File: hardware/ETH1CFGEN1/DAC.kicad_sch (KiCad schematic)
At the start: 42 parts, among them U601 TL072CD, U602 DAC8568IBPW, U603 TL072CD

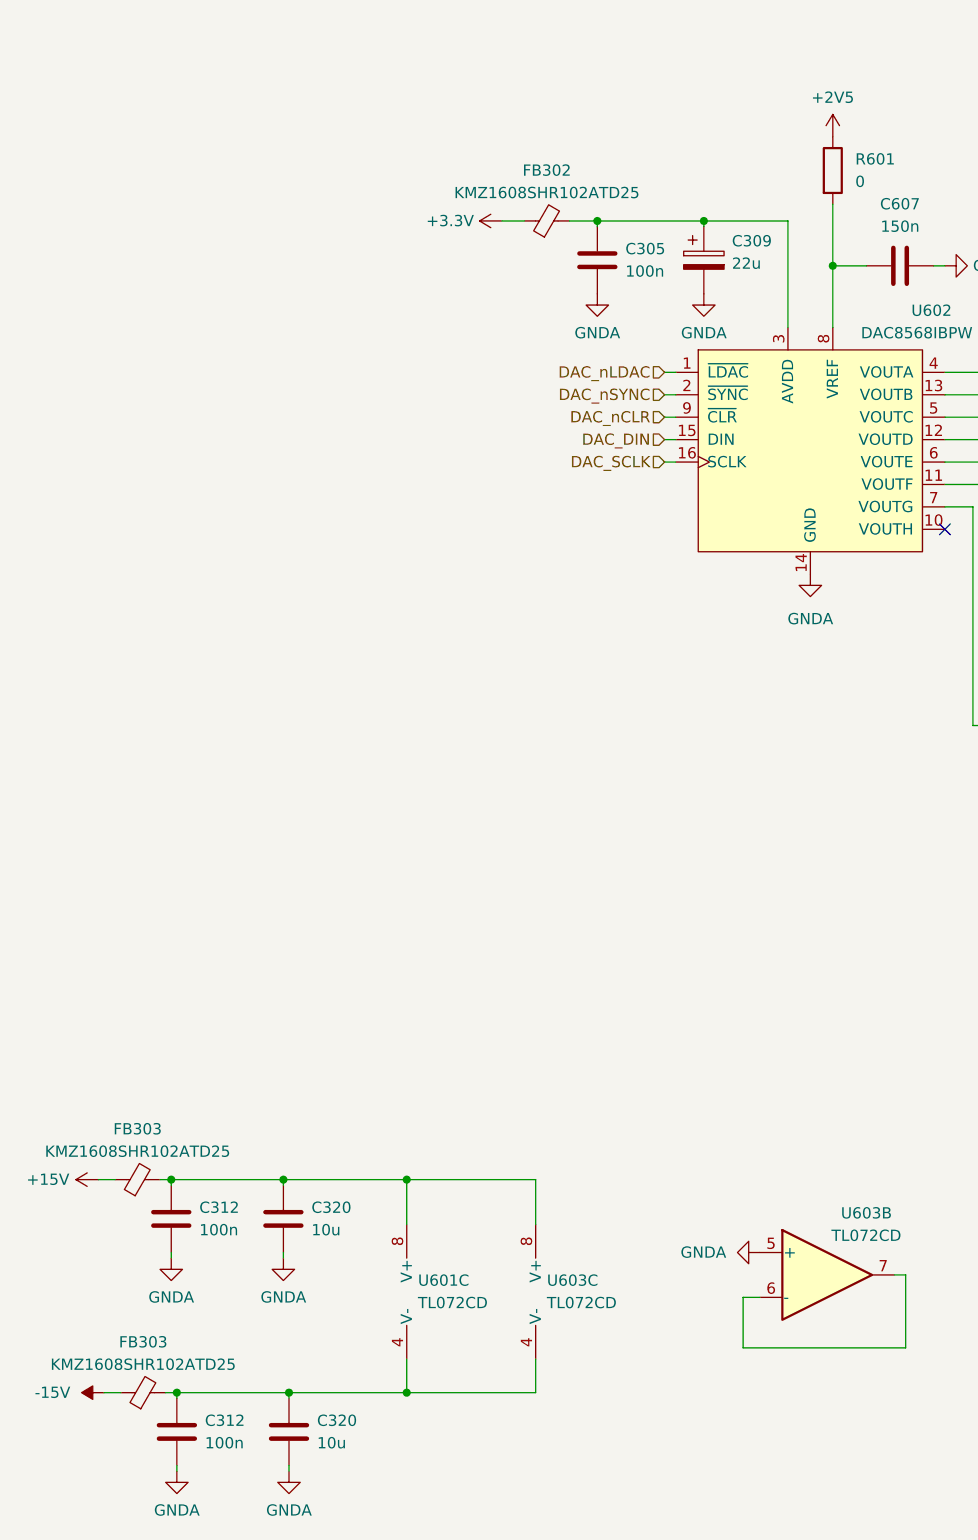
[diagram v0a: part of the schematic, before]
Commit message: PCB design
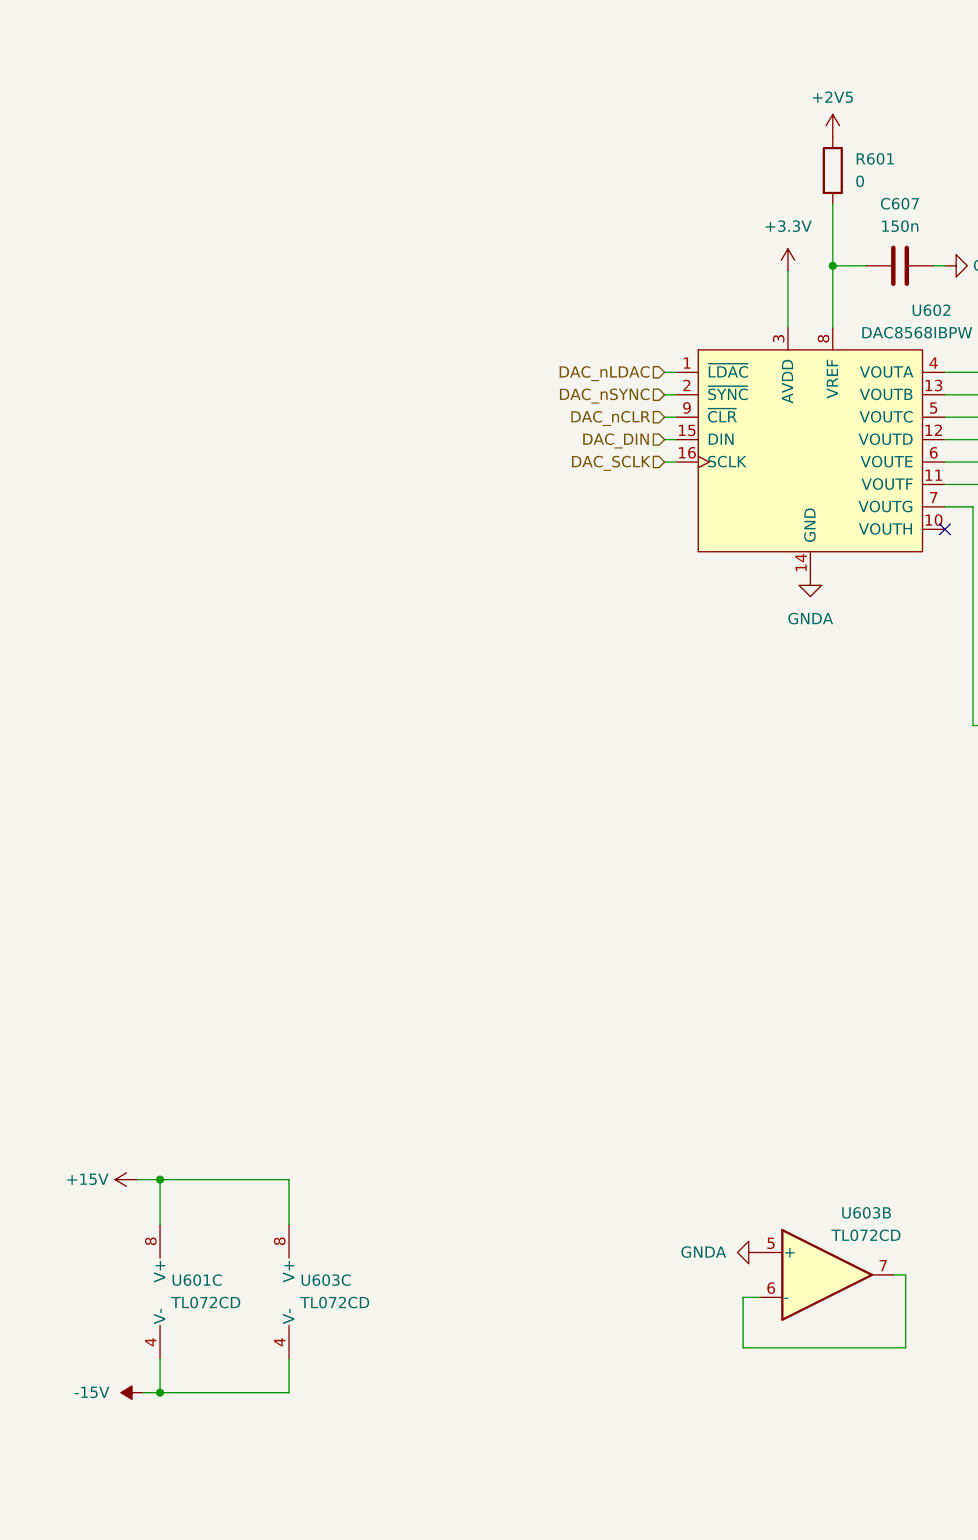
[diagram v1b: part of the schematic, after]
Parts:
- removed C305, C312 (x2): 100n, Capacitor_SMD:C_0603_1608Metric_Pad1.08x0.95mm_HandSolder, symbol Device:C
- removed C309: 22u, Capacitor_Tantalum_SMD:CP_EIA-7343-31_Kemet-D_Pad2.25x2.55mm_HandSolder, symbol Device:C_Polarized
- removed C320 (x2): 10u, Capacitor_SMD:C_1206_3216Metric_Pad1.33x1.80mm_HandSolder, symbol Device:C
- removed FB302, FB303 (x2): KMZ1608SHR102ATD25, Inductor_SMD:L_0603_1608Metric_Pad1.05x0.95mm_HandSolder, symbol Device:FerriteBead_Small
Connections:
- net +15V: now also U601.8 (V+), U603.8 (V+)
- net +3.3V: now also U602.3 (AVDD)
- net -15V: now also U601.4 (V-), U603.4 (V-)
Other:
- moved on the sheet: U601C, U603C
